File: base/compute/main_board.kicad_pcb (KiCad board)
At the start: 2 copper layers, 53.8 x 41.5 mm, 42 parts, among them J1 USB_C_Receptacle_USB2.0_16P, J2 Conn_01x20, J4 Conn_01x20, SW1 SW_Push_Open, SW2 SW_Push_Open, U1 MCP1700T-1202ETT, U2 ESP32-S3-WROOM-2, U3 LD1117S33TR_SOT223, U4 W25X20CLSN, U5 ICE40UP5K-SG48ITR-FPGA_Lattice

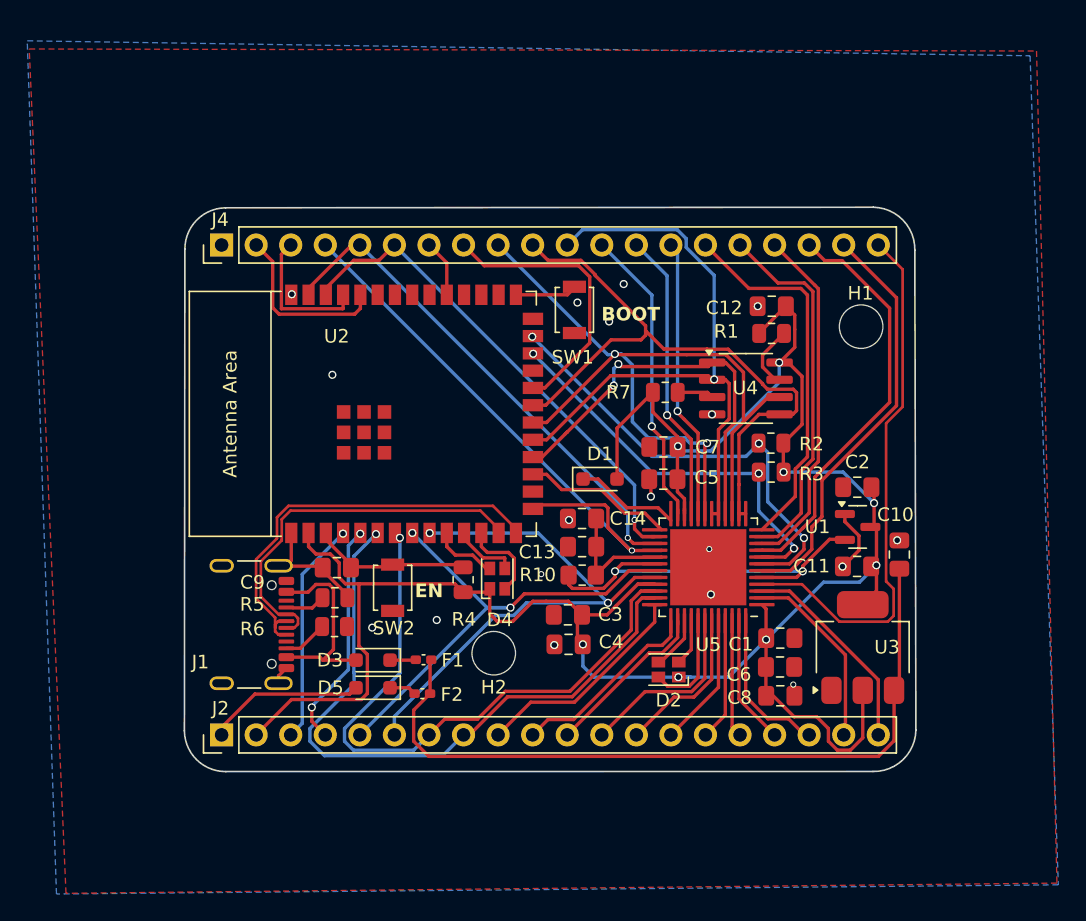
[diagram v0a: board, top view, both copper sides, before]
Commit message: improved layout main board
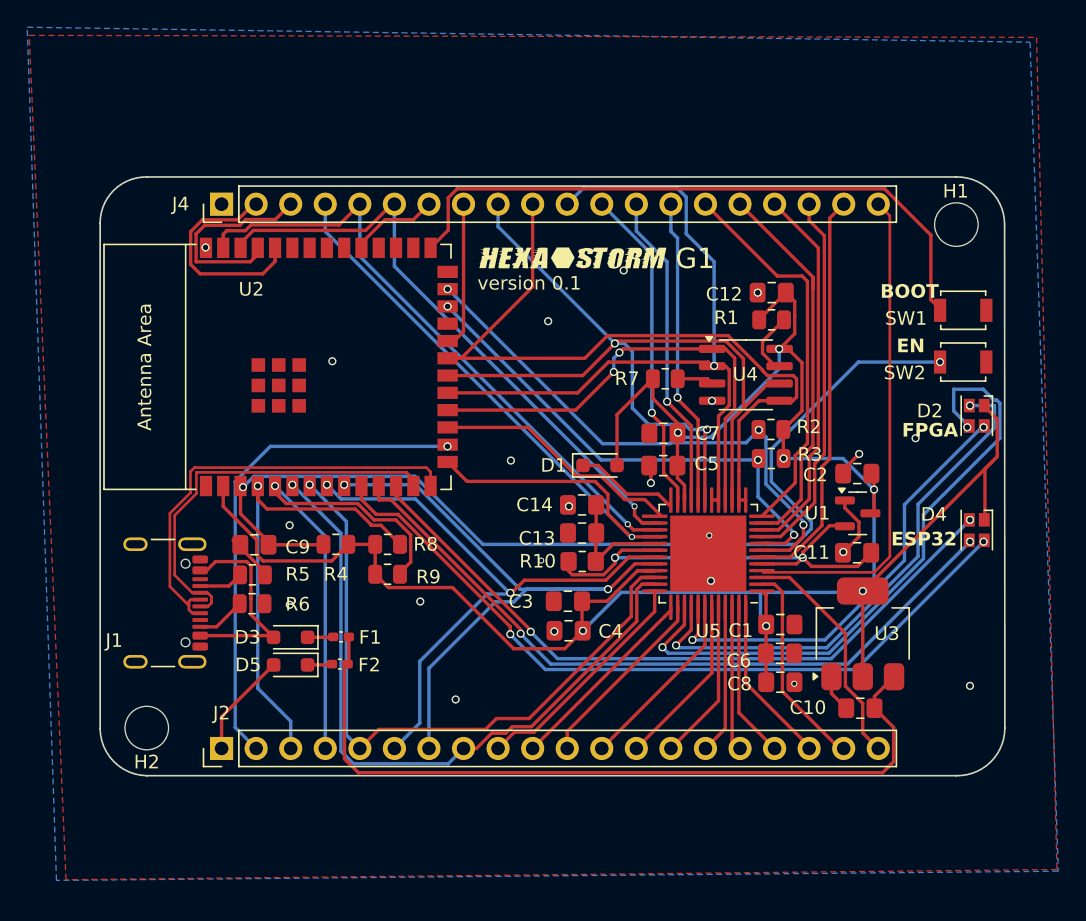
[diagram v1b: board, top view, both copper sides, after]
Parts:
- added R8: 10K, Resistor_SMD:R_0805_2012Metric, F.Cu at (192.2, 155.0)
- added R9: 10K, Resistor_SMD:R_0805_2012Metric, F.Cu at (192.2, 157.2)
- G1: moved to F.Cu
- moved SW2 45.1 mm to (234.5, 141.6), turned to 0 degrees
- moved D4 35.4 mm to (235.5, 153.9), turned to -90 degrees
- moved D2 29.3 mm to (235.5, 145.6), turned to -90 degrees
- moved SW1 28.6 mm to (234.5, 137.8), turned to 0 degrees
- moved H2 26.1 mm to (174.5, 168.5)
- moved C10 11.6 mm to (226.9, 167.0), turned to 180 degrees
- moved H1 10.3 mm to (234.0, 131.5)
- moved R4 9.70 mm to (188.4, 155.0), turned to 180 degrees
- moved G1 8.46 mm to (205.6, 133.8), turned to 0 degrees
- moved U2 7.16 mm to (187.1, 142.0)
- moved J1 6.53 mm to (174.7, 159.3)
- moved F2 6.44 mm to (188.7, 163.8)
- moved C9 6.29 mm to (182.4, 155.0)
- moved D3 6.29 mm to (185.1, 161.8)
- moved D5 6.29 mm to (185.1, 163.9)
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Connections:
- C11 pad 1: +3.3V -> +1V2
- J2 pad 2: +3.3V -> GPIO46
- J2 pad 5: FPGA42 -> FPGA44
- J2 pad 6: FPGA43 -> FPGA42
- J2 pad 7: FPGA44 -> FPGA43
- U2 pad 16: unconnected-(U2-GPIO46-Pad16) -> GPIO46
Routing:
- net Net-(U2-EN): track 12.2 -> 76.0 mm, vias 0 -> 2
- net ESP32_BLUE: track 4.83 -> 56.1 mm, vias 0 -> 2
- net ESP32_GREEN: track 4.76 -> 53.4 mm, vias 0 -> 2
- net ESP32_RED: track 6.32 -> 52.1 mm, vias 0 -> 2
- net FPGAG: track 4.43 -> 47.5 mm, vias 0 -> 2
- net Net-(U2-GPIO0/BOOT): track 4.51 -> 47.2 mm
- net GPIO46: track 0.00 -> 36.9 mm, vias 0 -> 1
- net FPGAB: track 3.91 -> 39.6 mm, vias 0 -> 2
- net FPGAR: track 8.13 -> 33.3 mm, vias 0 -> 2
- net POT_SCL: track 16.8 -> 35.8 mm, vias 2 -> 1
- net POT_SDA: track 16.4 -> 33.1 mm
- net SPI_SS_MOTOR: track 20.6 -> 10.8 mm
- net FPGA41: track 43.7 -> 52.7 mm
- net FPGA38: track 37.9 -> 46.3 mm
- net FPGA43: track 40.5 -> 48.8 mm
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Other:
- board size 53.8 x 41.5 mm -> 66.5 x 44 mm
- board text added: "ESP32"
- board text added: "FPGA"
- board text added: "version 0.1"
